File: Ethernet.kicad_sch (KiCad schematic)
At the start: 7 parts, among them J601 HC915320A-909-A, U601 RCLAMP0524P, U602 RCLAMP0524P

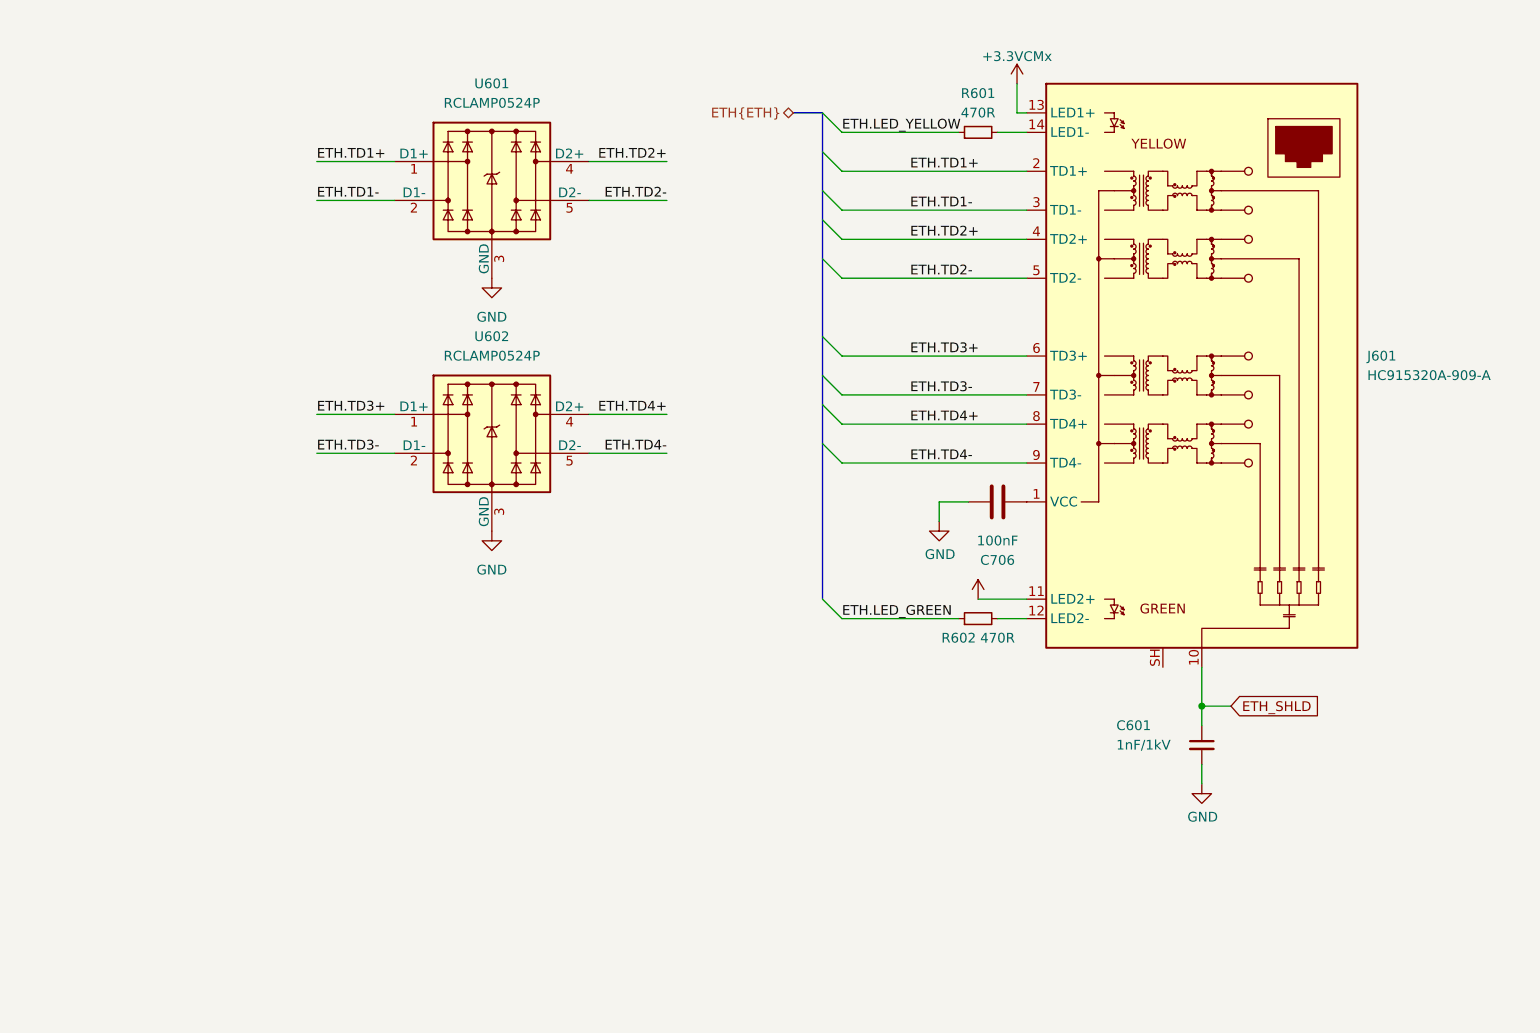
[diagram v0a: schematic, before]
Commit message: A big part of layout and routing done
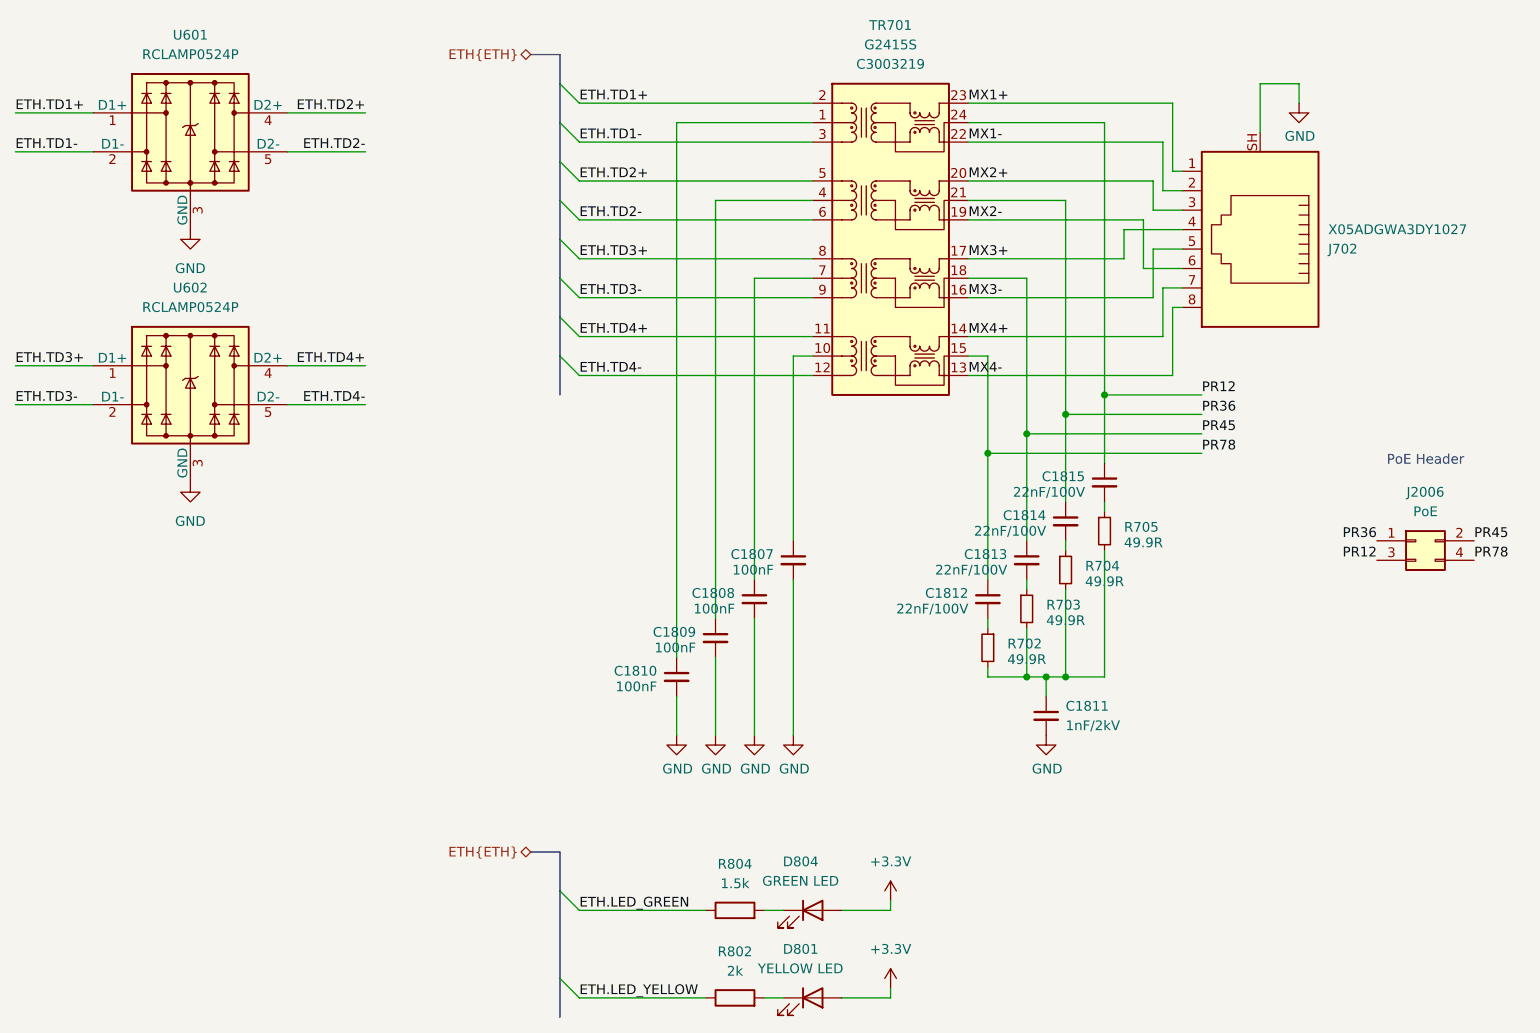
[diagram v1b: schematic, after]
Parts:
- removed C601: 1nF/1kV, Capacitor_SMD:C_1206_3216Metric, symbol Device:C_Small
- removed C706: 100nF, Capacitor_SMD:C_0402_1005Metric, symbol Device:C
- removed J601: HC915320A-909-A, Hatlabs:RJ45_HC915320A-909-A_Vertical, symbol Hatlabs:RJ45_HCTL_HC915320A-909-A_Vertical
- removed R601, R602: 470R, Resistor_SMD:R_0402_1005Metric, symbol Device:R_Small
- added C1807, C1808, C1809, C1810: 100nF, Capacitor_SMD:C_0402_1005Metric, symbol Device:C_Small
- added C1811: 1nF/2kV, Capacitor_SMD:C_1206_3216Metric, symbol Device:C_Small
- added C1812, C1813, C1814, C1815: 22nF/100V, Capacitor_SMD:C_0402_1005Metric, symbol Device:C_Small
- added D801: YELLOW LED, LED_SMD:LED_0603_1608Metric, symbol Device:LED
- added D804: GREEN LED, LED_SMD:LED_0603_1608Metric, symbol Device:LED
- added J2006: PoE, Connector_PinHeader_2.54mm:PinHeader_2x02_P2.54mm_Vertical, symbol Connector_Generic:Conn_02x02_Odd_Even
- added J702: X05ADGWA3DY1027, Hatlabs:RJ45-TH_XKB_X05ADGWA3DY1027, symbol Connector:RJ45_Shielded
- added R702, R703, R704, R705: 49.9R, Resistor_SMD:R_0402_1005Metric, symbol Device:R_Small
- added R802: 2k, Resistor_SMD:R_0402_1005Metric, symbol Device:R
- added R804: 1.5k, Resistor_SMD:R_0402_1005Metric, symbol Device:R
- added TR701: G2415S, Transformer_SMD:Transformer_Ethernet_YDS_30F-51NL_SO-24_7.1x15.1mm, symbol Transformer:30F-51NL
- U601: Component Class (none) -> fine_pitch; Manufacturer Texas Instruments -> (none); PartNumber TPD4EUSB30DQAR -> (none)
- U602: Component Class (none) -> fine_pitch; PartNumber TPD4EUSB30DQAR -> (none)
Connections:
- net ETH.LED_GREEN: now also R804.1
- net ETH.LED_YELLOW: now also R802.1
- net ETH.TD1+: now also TR701.2 (TD1+)
- net ETH.TD1-: now also TR701.3 (TD1-)
- net ETH.TD2+: now also TR701.5 (TD2+)
- net ETH.TD2-: now also TR701.6 (TD2-)
- net ETH.TD3+: now also TR701.8 (TD3+)
- net ETH.TD3-: now also TR701.9 (TD3-)
- net ETH.TD4+: now also TR701.11 (TD4+)
- net ETH.TD4-: now also TR701.12 (TD4-)
- net GND: now also C1807.2, C1808.2, C1809.2, C1810.2, C1811.2, J702.SH
- new net: D801.1 (K), R802.2
- new net: C1811.1, R702.2, R703.2, R704.2, R705.2
- new net: D804.1 (K), R804.2
- new net: C1807.1, TR701.10 (CT)
- new net: C1810.1, TR701.1 (CT)
- new net: C1809.1, TR701.4 (CT)
- new net: C1808.1, TR701.7 (CT)
- new net: C1815.2, R705.1
- new net: C1813.2, R703.1
- new net: C1812.2, R702.1
- new net: C1814.2, R704.1
- new net +3.3V: D801.2 (A), D804.2 (A)
- new net MX1+: J702.1, TR701.23 (MX1+)
- new net MX1-: J702.2, TR701.22 (MX1-)
- new net MX2+: J702.3, TR701.20 (MX2+)
- new net MX2-: J702.6, TR701.19 (MX2-)
- new net MX3+: J702.4, TR701.17 (MX3+)
- new net MX3-: J702.5, TR701.16 (MX3-)
- new net MX4+: J702.7, TR701.14 (MX4+)
- new net MX4-: J702.8, TR701.13 (MX4-)
- new net PR12: C1815.1, J2006.3 (Pin_3), TR701.24 (CT)
- new net PR36: C1814.1, J2006.1 (Pin_1), TR701.21 (CT)
- new net PR45: C1813.1, J2006.2 (Pin_2), TR701.18 (CT)
- new net PR78: C1812.1, J2006.4 (Pin_4), TR701.15 (CT)
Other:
- note added: "PoE Header"
- moved on the sheet: U601, U602
